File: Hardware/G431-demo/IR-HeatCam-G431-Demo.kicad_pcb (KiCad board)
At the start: 4 copper layers, 36 parts, among them J1 Conn_SDCard, J2 USB_C_Receptacle_USB2.0, J3 Conn_UART, J4 Conn_I2C, J5 Conn_ADC1, J6 Conn_ADC2, J7 Conn_01x18_MountingPin, J8 Conn_Touch, J9 SWD, U1 STM32G431CBUx, U2 RT9013-33GB, Y1 Crystal_GND24_12MHz

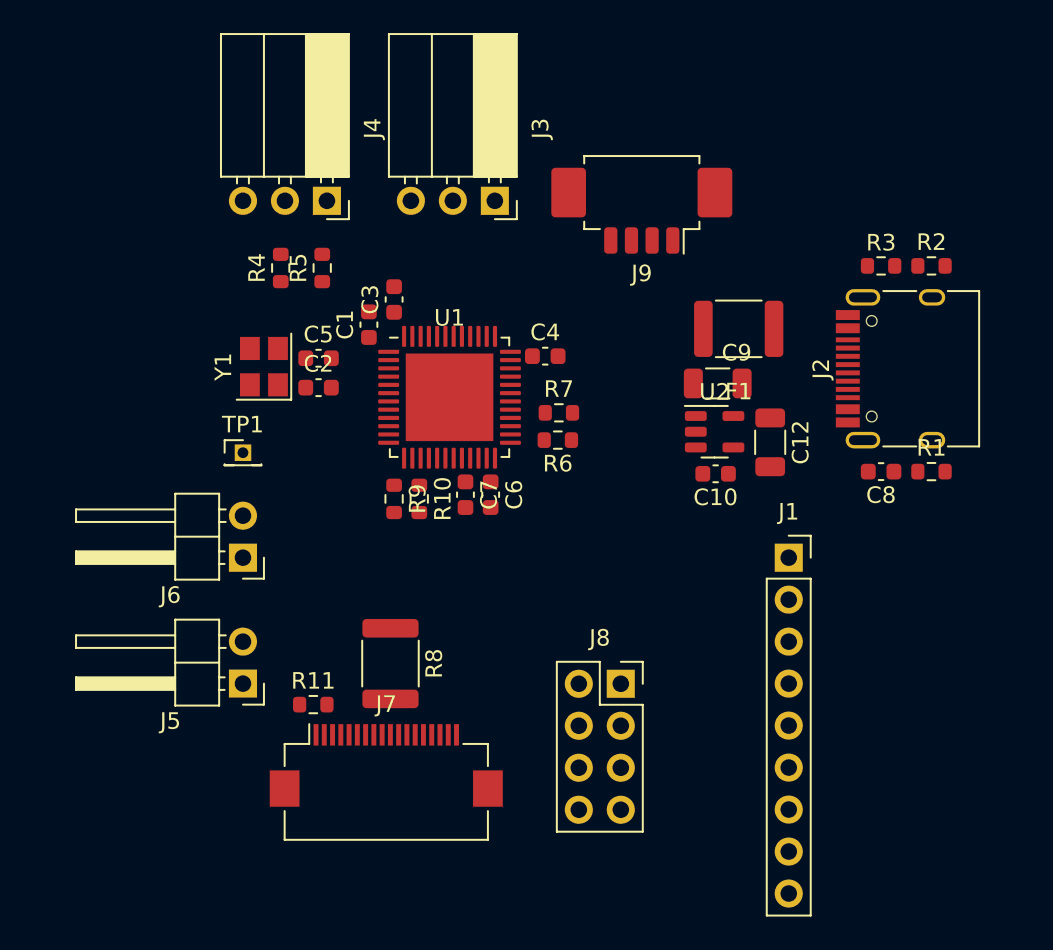
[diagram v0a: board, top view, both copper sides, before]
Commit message: pcb
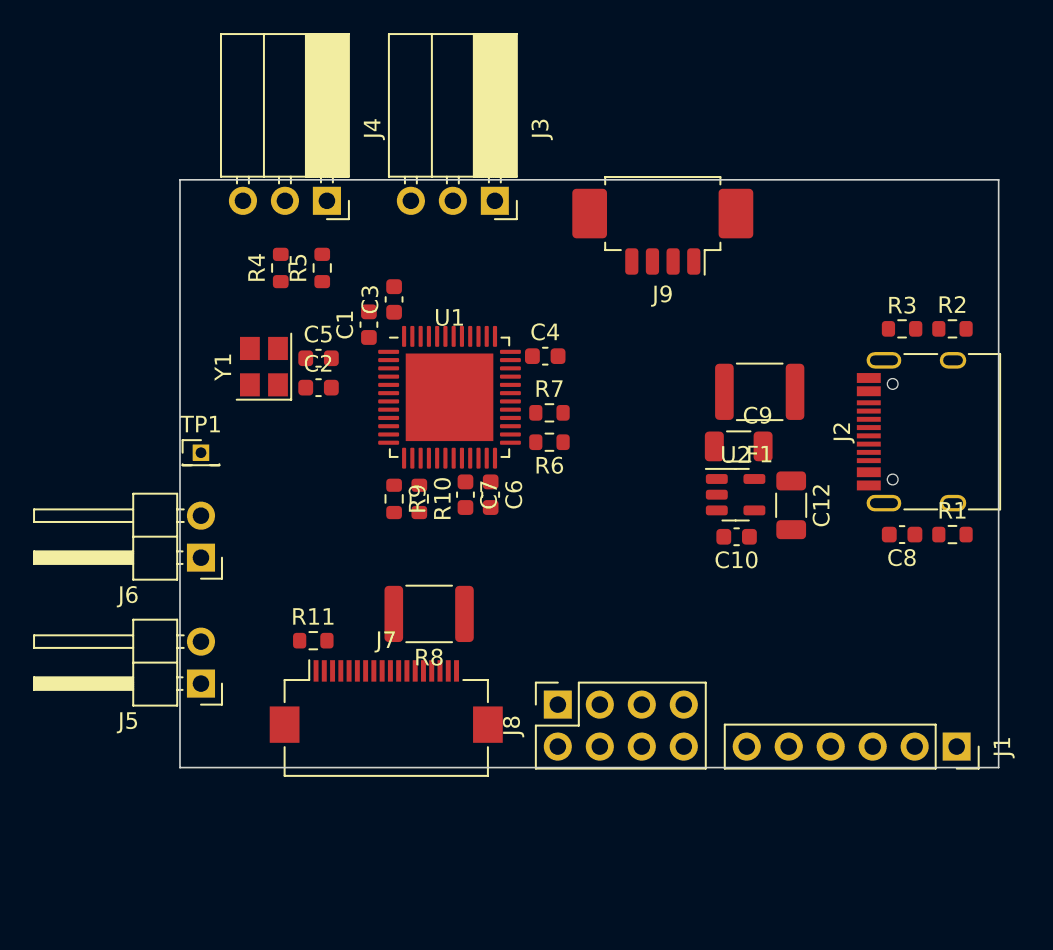
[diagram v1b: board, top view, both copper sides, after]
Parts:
- J1: footprint Connector_PinSocket_2.54mm:PinSocket_1x09_P2.54mm_Vertical -> Connector_PinSocket_2.54mm:PinSocket_1x06_P2.54mm_Vertical
- moved J1 15.3 mm to (108.0, 146.1), turned to -90 degrees
- moved F1 4.02 mm to (96.0, 124.6)
- moved J2 4.02 mm to (106.7, 127.0)
- moved U2 4.02 mm to (94.6, 130.8)
- moved C10 4.02 mm to (94.6, 133.4)
- moved C8 4.02 mm to (104.6, 133.2)
- moved C9 4.02 mm to (94.8, 127.9)
- moved R1 4.02 mm to (107.7, 133.2)
- moved R2 4.02 mm to (107.7, 120.8)
- moved R3 4.02 mm to (104.6, 120.8)
- moved C12 4.02 mm to (97.9, 131.5)
- moved J8 4.01 mm to (83.8, 143.5), turned to 90 degrees
- moved J7 3.87 mm to (73.4, 143.3)
- moved R11 3.87 mm to (69.0, 139.6)
- moved R8 3.81 mm to (76.0, 138.0), turned to 180 degrees
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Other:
- board outline added: 49.5 x 35.6 mm
